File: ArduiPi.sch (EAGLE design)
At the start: 101 parts, among them IC1 AVR-MEGA8-PPTH, IC2 DS2482-100S, J11 DNP, J12 DNP, J13 DNP, J14 Teleinfo, J2 DNP, J3 DNP, J4 DNP, J5 DNP, J6 DNP, J7 DNP, J8 DNP, J9 DC-044-AH, Q1 BSS138, Q2 BSS138, Q3 BSS138, Q4 BSS138, Q5 BSS84, Q6 BSS138, Q7 BSS138, U1 78M05, U2 LD1117 3V3, U3 TXB0104, U4 TXB0108, U5 TXB0108, X1 16Mhz

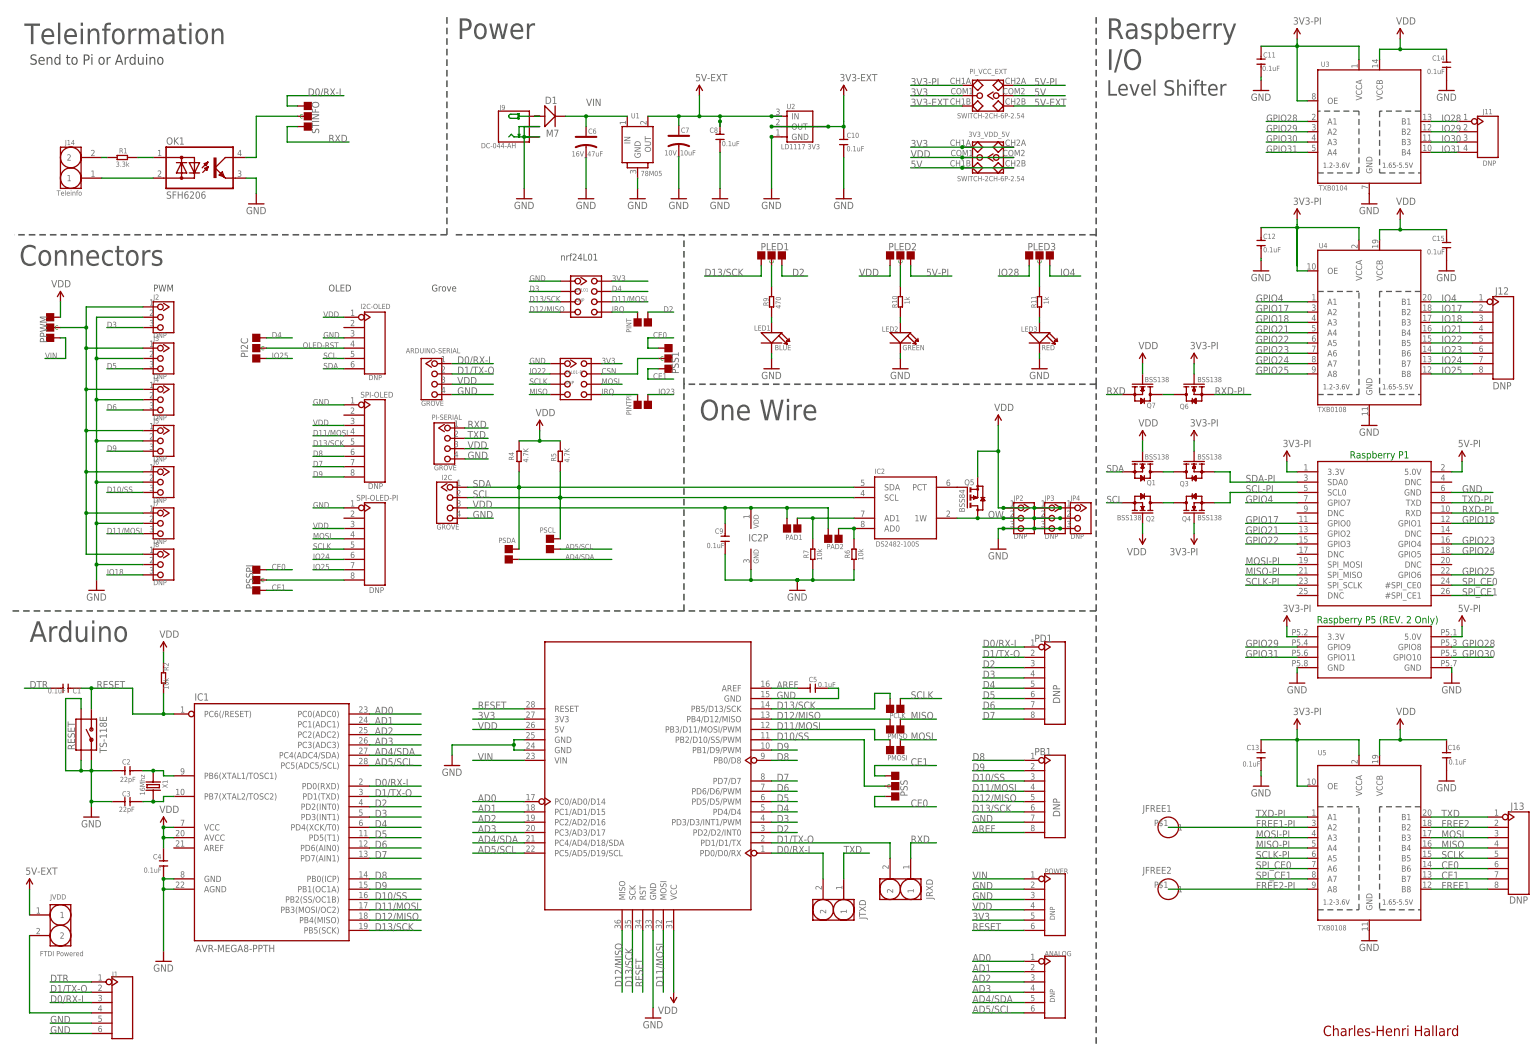
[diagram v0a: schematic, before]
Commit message: ArduiPi Production Version V0.9d
ArduiPi Production Version V0.9d
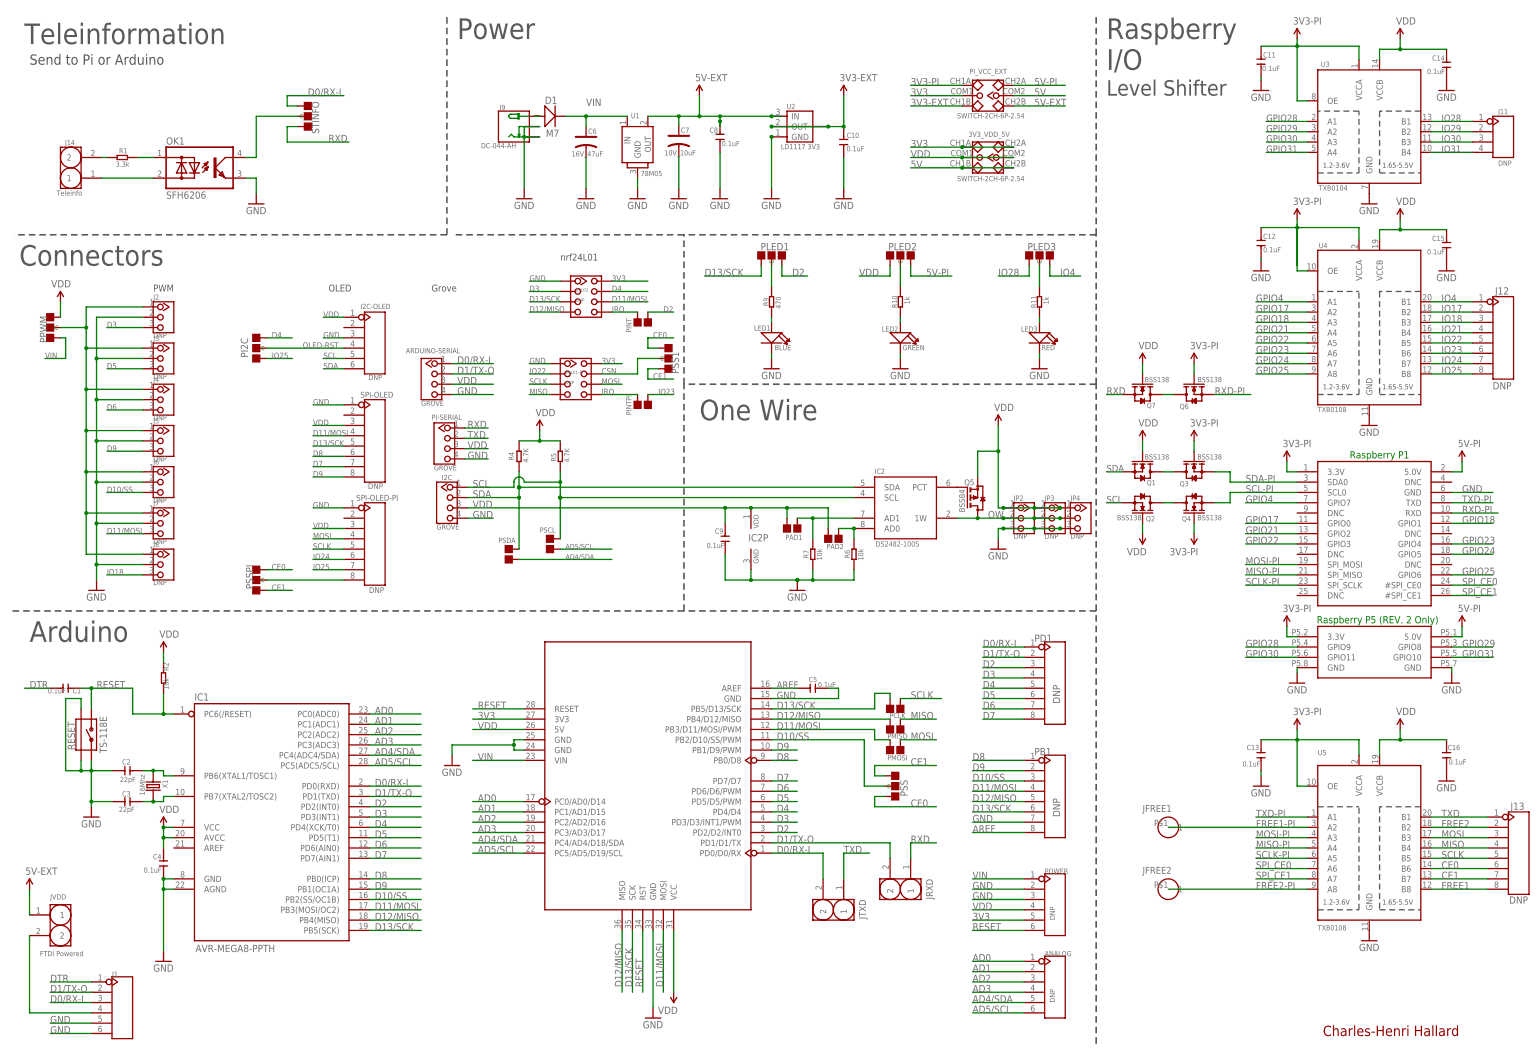
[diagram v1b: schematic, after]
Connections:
- net GPIO28: now also PI-P1.GPIO9; no longer PI-P1.GPIO8
- net GPIO29: now also PI-P1.GPIO8; no longer PI-P1.GPIO9
- net GPIO30: now also PI-P1.GPIO11; no longer PI-P1.GPIO10
- net GPIO31: now also PI-P1.GPIO10; no longer PI-P1.GPIO11
- net SCL: now also I2C.1; no longer I2C.2
- net SDA: now also I2C.2; no longer I2C.1
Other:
- moved on the sheet: J11
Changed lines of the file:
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@@
 <?xml version="1.0" encoding="utf-8"?>
 <!DOCTYPE eagle SYSTEM "eagle.dtd">
-<eagle version="6.3">
+<eagle version="6.4">
 <drawing>
 <settings>
@@
 <setting verticaltext="up"/>
 </settings>
-<grid distance="0.1" unitdist="inch" unit="inch" style="lines" multiple="1" display="no" altdistance="0.01" altunitdist="inch" altunit="inch"/>
+<grid distance="50" unitdist="mil" unit="mil" style="lines" multiple="1" display="yes" altdistance="25" altunitdist="mil" altunit="mil"/>
 <layers>
 <layer number="1" name="Top" color="4" fill="1" visible="no" active="no"/>
@@
 </instance>
 <instance part="GND26" gate="1" x="363.22" y="172.72"/>
-<instance part="J11" gate="G$1" x="392.43" y="189.23" smashed="yes">
-<attribute name="NAME" x="391.16" y="194.818" size="1.27" layer="95"/>
-<attribute name="VALUE" x="391.16" y="182.118" size="1.27" layer="96"/>
+<instance part="J11" gate="G$1" x="396.24" y="189.23" smashed="yes">
+<attribute name="NAME" x="394.97" y="194.818" size="1.27" layer="95"/>
+<attribute name="VALUE" x="394.97" y="182.118" size="1.27" layer="96"/>
 </instance>
 <instance part="Q5" gate="G$1" x="266.7" y="100.33" smashed="yes">
@@
 <segment>
 <pinref part="IC2" gate="G$1" pin="SCL"/>
-<label x="142.24" y="100.33" size="1.778" layer="95"/>
-<pinref part="I2C" gate="G$1" pin="2"/>
+<label x="142.24" y="102.87" size="1.778" layer="95"/>
 <pinref part="PSCL" gate="G$1" pin="2"/>
 <wire x1="236.22" y1="100.33" x2="163.83" y2="100.33" width="0.1524" layer="91"/>
-<wire x1="163.83" y1="100.33" x2="140.97" y2="100.33" width="0.1524" layer="91"/>
 <wire x1="163.83" y1="90.17" x2="163.83" y2="100.33" width="0.1524" layer="91"/>
 <junction x="163.83" y="100.33"/>
 <junction x="163.83" y="100.33"/>
-<wire x1="163.83" y1="106.68" x2="163.83" y2="100.33" width="0.1524" layer="91"/>
+<wire x1="163.83" y1="106.68" x2="163.83" y2="104.14" width="0.1524" layer="91"/>
 <pinref part="R5" gate="R" pin="1"/>
+<pinref part="I2C" gate="G$1" pin="1"/>
+<wire x1="163.83" y1="104.14" x2="163.83" y2="100.33" width="0.1524" layer="91"/>
+<wire x1="140.97" y1="102.87" x2="152.4" y2="102.87" width="0.1524" layer="91"/>
+<wire x1="152.4" y1="102.87" x2="152.4" y2="104.14" width="0.1524" layer="91"/>
+<wire x1="152.4" y1="104.14" x2="153.67" y2="105.41" width="0.1524" layer="91" curve="-90"/>
+<wire x1="153.67" y1="105.41" x2="154.94" y2="104.14" width="0.1524" layer="91" curve="-90"/>
+<wire x1="154.94" y1="104.14" x2="163.83" y2="104.14" width="0.1524" layer="91"/>
+<junction x="163.83" y="104.14"/>
 </segment>
 <segment>
@@
 <segment>
 <pinref part="IC2" gate="G$1" pin="SDA"/>
-<label x="142.24" y="102.87" size="1.778" layer="95"/>
-<pinref part="I2C" gate="G$1" pin="1"/>
+<label x="142.24" y="100.33" size="1.778" layer="95"/>
 <pinref part="PSDA" gate="G$1" pin="2"/>
 <wire x1="236.22" y1="102.87" x2="153.67" y2="102.87" width="0.1524" layer="91"/>
-<wire x1="153.67" y1="102.87" x2="140.97" y2="102.87" width="0.1524" layer="91"/>
-<wire x1="153.67" y1="87.63" x2="153.67" y2="102.87" width="0.1524" layer="91"/>
+<wire x1="153.67" y1="87.63" x2="153.67" y2="100.33" width="0.1524" layer="91"/>
 <junction x="153.67" y="102.87"/>
 <junction x="153.67" y="102.87"/>
+<wire x1="153.67" y1="100.33" x2="153.67" y2="102.87" width="0.1524" layer="91"/>
 <wire x1="153.67" y1="106.68" x2="153.67" y2="102.87" width="0.1524" layer="91"/>
 <pinref part="R4" gate="R" pin="1"/>
+<pinref part="I2C" gate="G$1" pin="2"/>
+<wire x1="140.97" y1="100.33" x2="153.67" y2="100.33" width="0.1524" layer="91"/>
+<junction x="153.67" y="100.33"/>
 </segment>
 <segment>
@@
 <net name="GPIO28" class="0">
 <segment>
+<pinref part="U3" gate="G$1" pin="A1"/>
+<wire x1="347.98" y1="193.04" x2="337.82" y2="193.04" width="0.1524" layer="91"/>
+<label x="337.82" y="193.04" size="1.6764" layer="95"/>
+</segment>
+<segment>
+<wire x1="345.44" y1="63.5" x2="332.74" y2="63.5" width="0.1524" layer="91"/>
+<label x="332.74" y="63.5" size="1.778" layer="95"/>
+<pinref part="PI-P1" gate="G$1" pin="GPIO9"/>
+</segment>
+</net>
+<net name="GPIO30" class="0">
+<segment>
+<pinref part="U3" gate="G$1" pin="A3"/>
+<wire x1="347.98" y1="187.96" x2="337.82" y2="187.96" width="0.1524" layer="91"/>
+<label x="337.82" y="187.96" size="1.6764" layer="95"/>
+</segment>
+<segment>
+<wire x1="345.44" y1="60.96" x2="332.74" y2="60.96" width="0.1524" layer="91"/>
+<label x="332.74" y="60.96" size="1.778" layer="95"/>
+<pinref part="PI-P1" gate="G$1" pin="GPIO11"/>
+</segment>
+</net>
+<net name="GPIO29" class="0">
+<segment>
+<pinref part="U3" gate="G$1" pin="A2"/>
+<wire x1="347.98" y1="190.5" x2="337.82" y2="190.5" width="0.1524" layer="91"/>
+<label x="337.82" y="190.5" size="1.6764" layer="95"/>
+</segment>
+<segment>
 <wire x1="383.54" y1="63.5" x2="393.7" y2="63.5" width="0.1524" layer="91"/>
 <label x="386.08" y="63.5" size="1.778" layer="95"/>
 <pinref part="PI-P1" gate="G$1" pin="GPIO8"/>
 </segment>
-<segment>
-<pinref part="U3" gate="G$1" pin="A1"/>
-<wire x1="347.98" y1="193.04" x2="337.82" y2="193.04" width="0.1524" layer="91"/>
-<label x="337.82" y="193.04" size="1.6764" layer="95"/>
-</segment>
-</net>
-<net name="GPIO30" class="0">
+</net>
+<net name="GPIO31" class="0">
+<segment>
+<pinref part="U3" gate="G$1" pin="A4"/>
+<wire x1="347.98" y1="185.42" x2="337.82" y2="185.42" width="0.1524" layer="91"/>
+<label x="337.82" y="185.42" size="1.6764" layer="95"/>
+</segment>
 <segment>
 <wire x1="383.54" y1="60.96" x2="393.7" y2="60.96" width="0.1524" layer="91"/>
 <label x="386.08" y="60.96" size="1.778" layer="95"/>
 <pinref part="PI-P1" gate="G$1" pin="GPIO10"/>
-</segment>
-<segment>
-<pinref part="U3" gate="G$1" pin="A3"/>
-<wire x1="347.98" y1="187.96" x2="337.82" y2="187.96" width="0.1524" layer="91"/>
-<label x="337.82" y="187.96" size="1.6764" layer="95"/>
-</segment>
-</net>
-<net name="GPIO29" class="0">
-<segment>
-<wire x1="345.44" y1="63.5" x2="332.74" y2="63.5" width="0.1524" layer="91"/>
-<label x="332.74" y="63.5" size="1.778" layer="95"/>
-<pinref part="PI-P1" gate="G$1" pin="GPIO9"/>
-</segment>
-<segment>
-<pinref part="U3" gate="G$1" pin="A2"/>
-<wire x1="347.98" y1="190.5" x2="337.82" y2="190.5" width="0.1524" layer="91"/>
-<label x="337.82" y="190.5" size="1.6764" layer="95"/>
-</segment>
-</net>
-<net name="GPIO31" class="0">
-<segment>
-<wire x1="345.44" y1="60.96" x2="332.74" y2="60.96" width="0.1524" layer="91"/>
-<label x="332.74" y="60.96" size="1.778" layer="95"/>
-<pinref part="PI-P1" gate="G$1" pin="GPIO11"/>
-</segment>
-<segment>
-<pinref part="U3" gate="G$1" pin="A4"/>
-<wire x1="347.98" y1="185.42" x2="337.82" y2="185.42" width="0.1524" layer="91"/>
-<label x="337.82" y="185.42" size="1.6764" layer="95"/>
 </segment>
 </net>
@@
 <segment>
 <pinref part="U3" gate="G$1" pin="B1"/>
-<wire x1="378.46" y1="193.04" x2="384.81" y2="193.04" width="0.1524" layer="91"/>
+<wire x1="378.46" y1="193.04" x2="388.62" y2="193.04" width="0.1524" layer="91"/>
 <label x="381" y="193.04" size="1.6764" layer="95"/>
 <pinref part="J11" gate="G$1" pin="P$1"/>
@@
 <segment>
 <pinref part="U3" gate="G$1" pin="B2"/>
-<wire x1="384.81" y1="190.5" x2="378.46" y2="190.5" width="0.1524" layer="91"/>
+<wire x1="388.62" y1="190.5" x2="378.46" y2="190.5" width="0.1524" layer="91"/>
 <label x="381" y="190.5" size="1.6764" layer="95"/>
 <pinref part="J11" gate="G$1" pin="P$2"/>
@@
 <segment>
 <pinref part="U3" gate="G$1" pin="B3"/>
-<wire x1="384.81" y1="187.96" x2="378.46" y2="187.96" width="0.1524" layer="91"/>
+<wire x1="388.62" y1="187.96" x2="378.46" y2="187.96" width="0.1524" layer="91"/>
 <label x="381" y="187.96" size="1.6764" layer="95"/>
 <pinref part="J11" gate="G$1" pin="P$3"/>
@@
 <segment>
 <pinref part="U3" gate="G$1" pin="B4"/>
-<wire x1="384.81" y1="185.42" x2="378.46" y2="185.42" width="0.1524" layer="91"/>
+<wire x1="388.62" y1="185.42" x2="378.46" y2="185.42" width="0.1524" layer="91"/>
 <label x="381" y="185.42" size="1.6764" layer="95"/>
 <pinref part="J11" gate="G$1" pin="P$4"/>
